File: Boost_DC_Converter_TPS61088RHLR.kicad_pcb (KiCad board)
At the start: 2 copper layers, 52.8 x 25.5 mm, 25 parts, among them P1 DG301-5.0-02P-12-00A(H), P2 DG301-5.0-02P-12-00A(H), P3 DG301-5.0-02P-12-00A(H), U1 RHL0020A

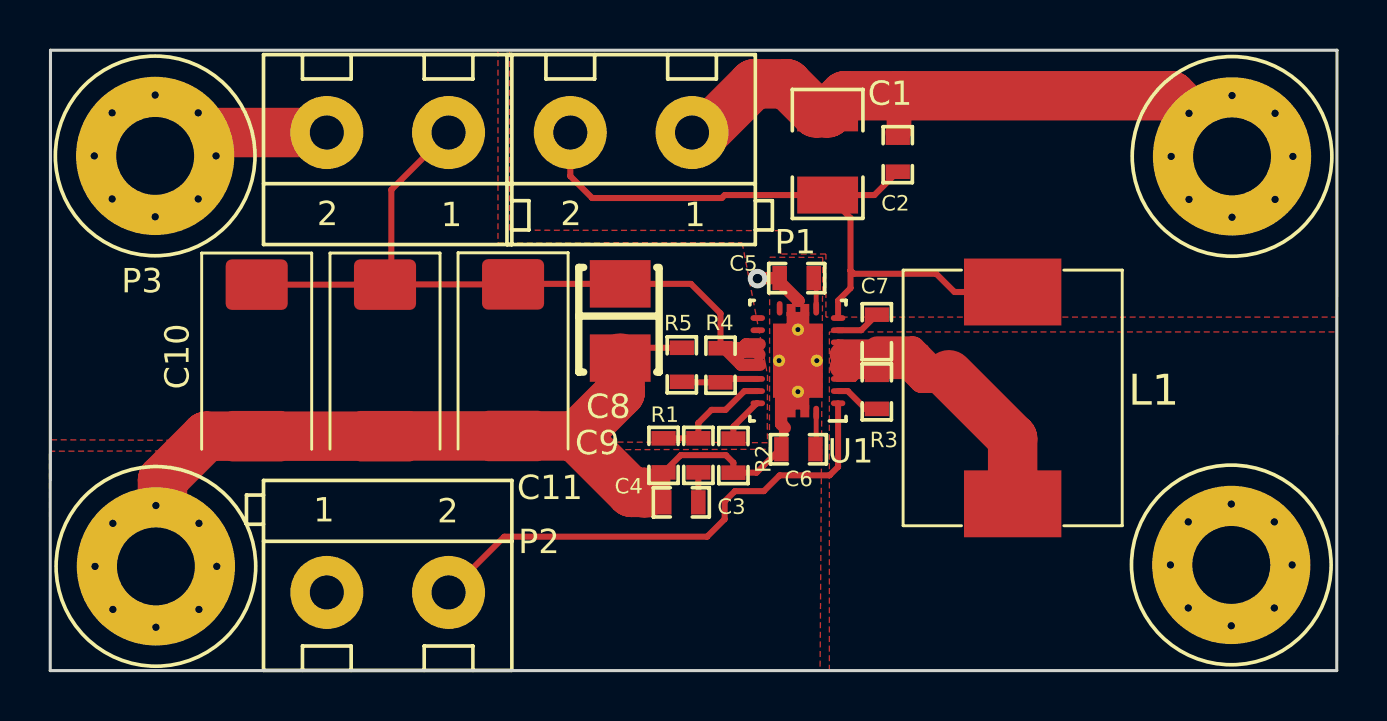
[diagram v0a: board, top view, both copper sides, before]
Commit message: Generated gerbers and schematic BOM
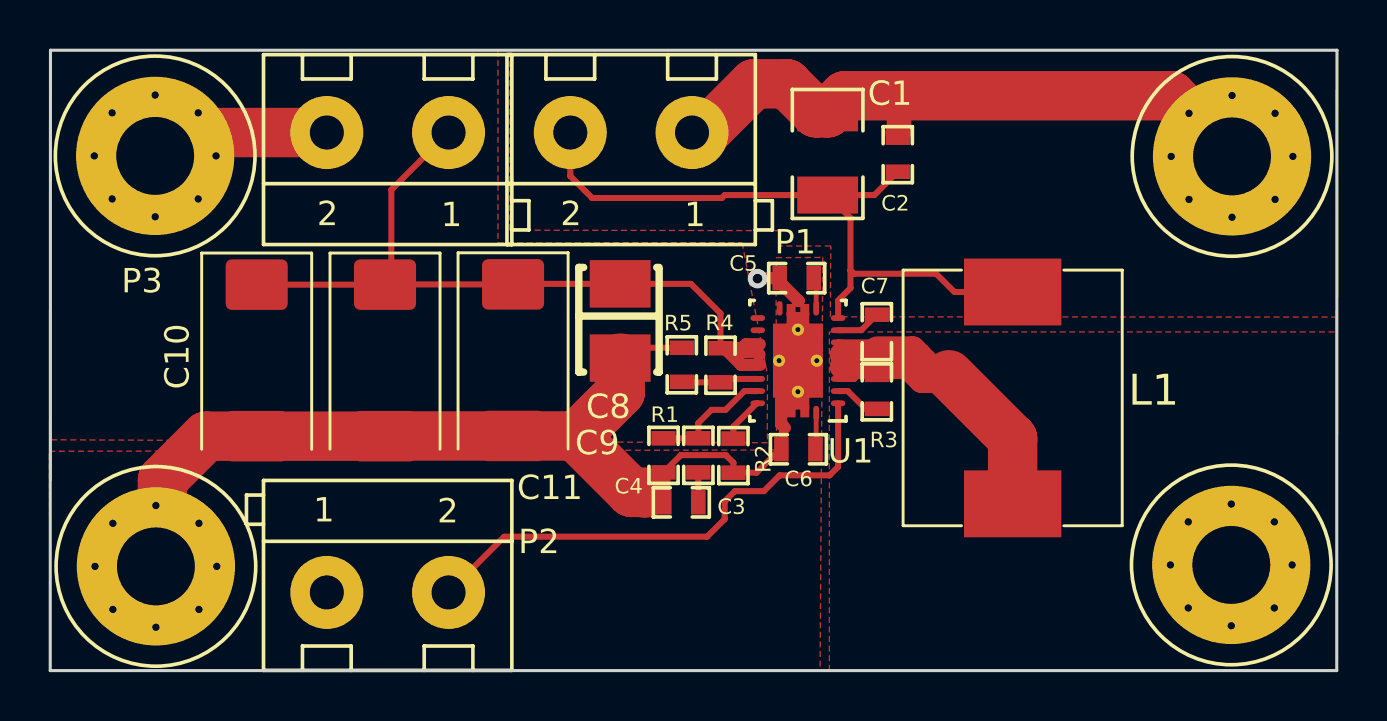
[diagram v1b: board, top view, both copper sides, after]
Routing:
- net GND: track 84.4 -> 88.6 mm
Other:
- net class GND added: clearance 0.152, trace_width 0.127, via_dia 0.8, via_drill 0.4
- rule trace_min: 0.2 -> 0.1
- rule via_min_drill: 0.3 -> 0.1
- rule via_min_size: 0.4 -> 0.1
